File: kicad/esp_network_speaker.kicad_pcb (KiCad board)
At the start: 2 copper layers, 50 parts, among them Q1 Q_NPN_BEC, Q2 Q_NPN_BEC, SW1 SW_PUSH, SW2 SW_PUSH, U1 23LC1024, U2 ESP12, U3 PCM5100A, U4 TSR_1-2433, U5 M74VHC1GT125

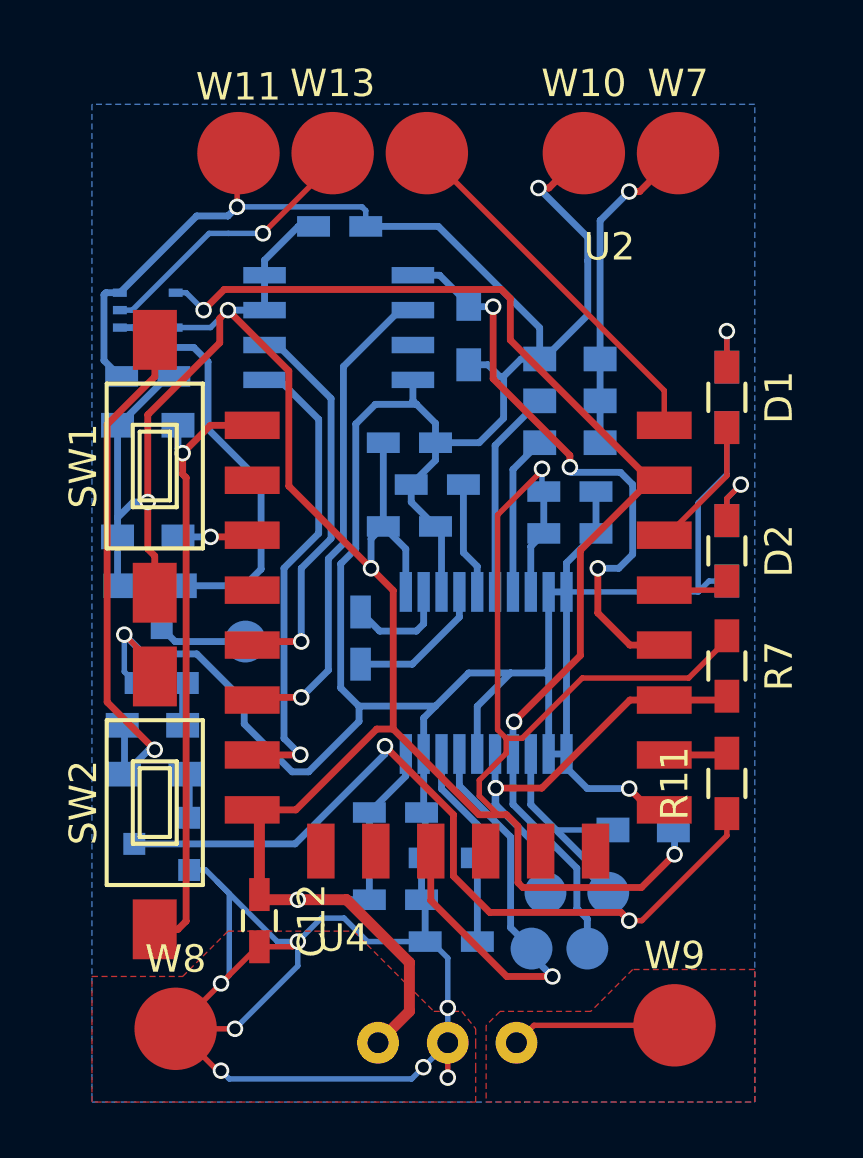
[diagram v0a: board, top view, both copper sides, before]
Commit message: wip, gerber files generated for rev A
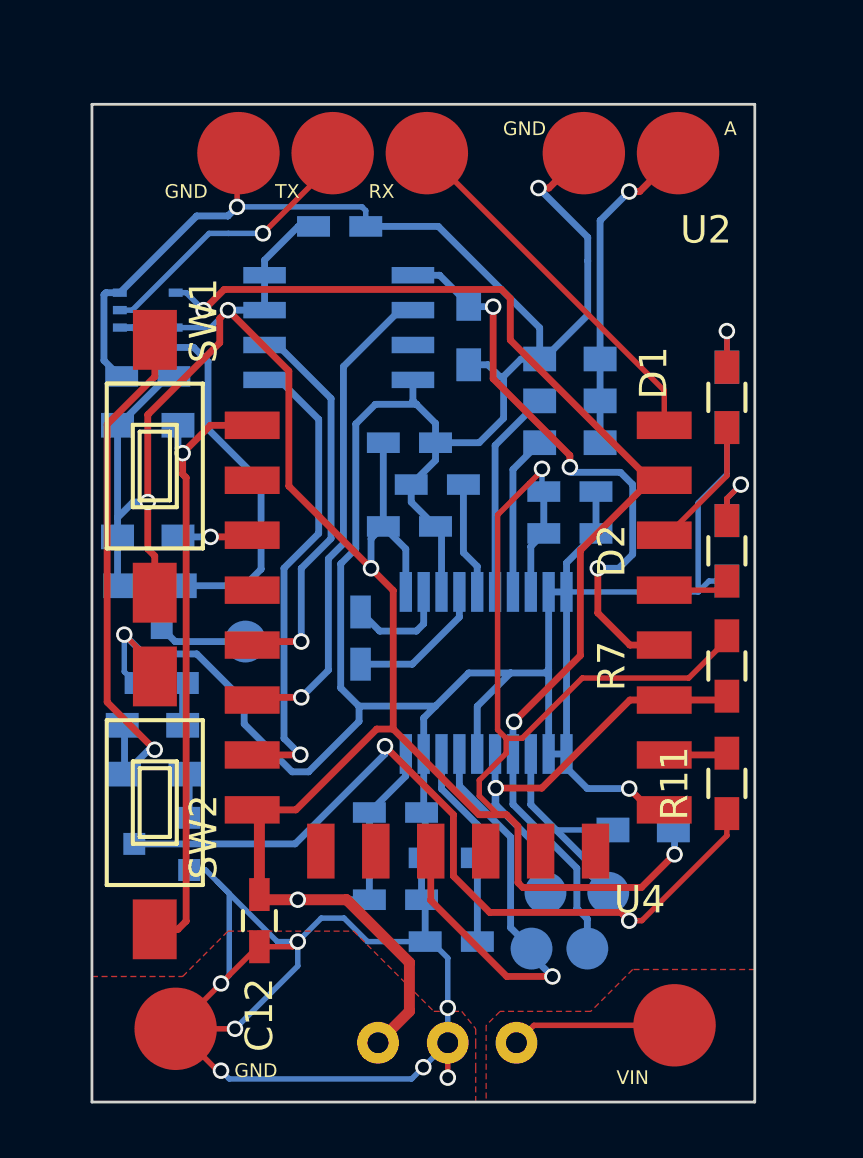
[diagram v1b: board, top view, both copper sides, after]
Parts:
- renumbered W2 to BCK, W4 to DTA, W3 to LRK, W5 to MTE, W1 to PRGEN
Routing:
- net (no net): track 0.00 -> 3.17 mm
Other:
- board outline added: 24.1 x 36.3 mm
- board text added: "A"
- board text added: "ESP12 NETWORK SPEAKER"
- board text added: "GND"
- board text added: "RX"
- board text added: "TX"
- board text added: "VIN"
- board text added: "https://github.com/JDRobotter/esp8266_network_speaker"
